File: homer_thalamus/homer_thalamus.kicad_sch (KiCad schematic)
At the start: 20 parts, among them J1 GPIO, J2 MotDrv_Pow_Conn, J3 Right_Motor_Conn, J4 Left_Motor_Conn, J5 Spare_GP_Conn, J6 VBUS_Conn, SW1 SW_PULLDOWN, U1 DRV8874_CARRIER_RIGHT, U2 DRV8874_CARRIER_LEFT, U3 HC-SR04

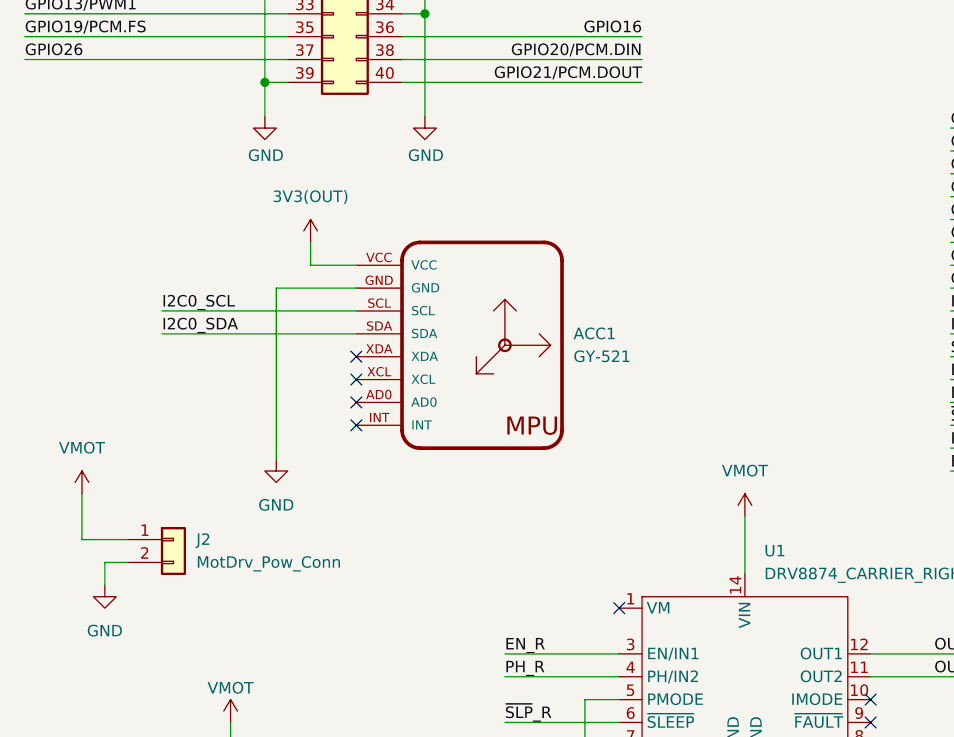
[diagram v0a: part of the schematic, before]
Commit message: update pcb layout
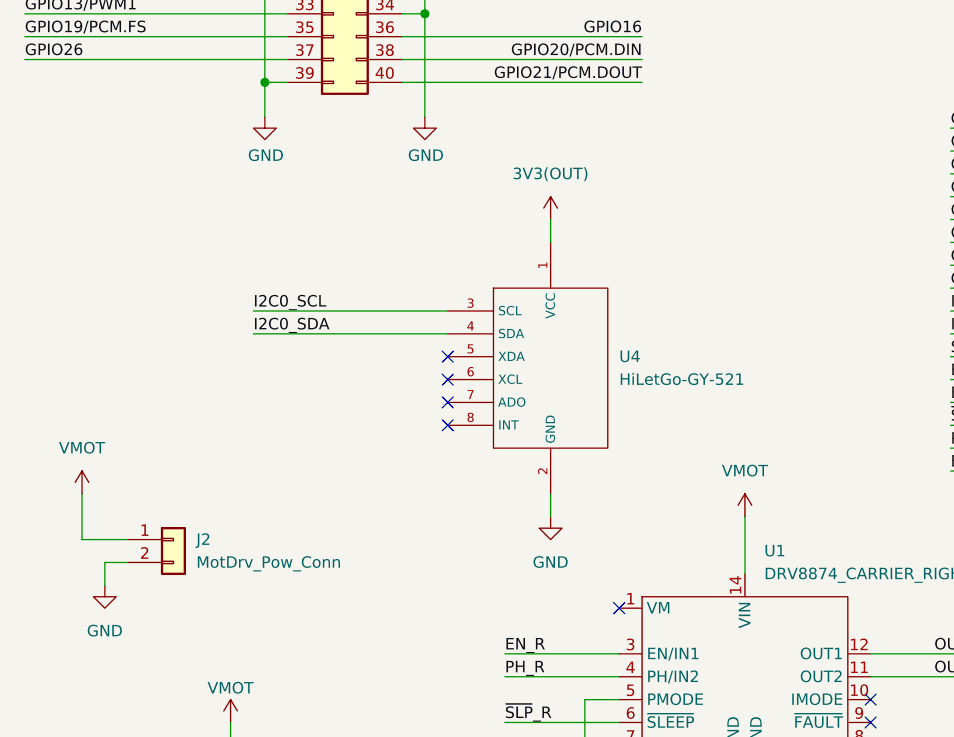
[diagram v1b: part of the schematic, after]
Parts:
- removed ACC1: GY-521, GY-521:GY-521, symbol GY-521:GY-521
- added U4: HiLetGo-GY-521, GY-521:HiLetGo-GY-521, symbol GY-521:HiLetGo-GY-521
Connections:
- net 3V3(OUT): now also U4.1 (VCC)
- net GND: now also U4.2 (GND)
- net I2C0_SCL: now also U4.3 (SCL)
- net I2C0_SDA: now also U4.4 (SDA)
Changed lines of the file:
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@@
 	)
 	(no_connect
-		(at 58.42 111.76)
+		(at 68.58 111.76)
 	)
 	(no_connect
@@
 	)
 	(no_connect
-		(at 58.42 109.22)
+		(at 68.58 109.22)
 	)
 	(no_connect
@@
 	)
 	(no_connect
-		(at 58.42 104.14)
+		(at 68.58 104.14)
 	)
 	(no_connect
@@
 	)
 	(no_connect
-		(at 58.42 106.68)
+		(at 68.58 106.68)
 	)
 	(no_connect
@@
 	(wire
 		(pts
-			(xy 58.42 96.52) (xy 49.53 96.52)
-		)
-		(stroke
-			(width 0)
-			(type default)
-		)
-	)
-	(wire
-		(pts
 			(xy 63.5 53.34) (xy 90.17 53.34)
 		)
@@
 	(wire
 		(pts
-			(xy 49.53 96.52) (xy 49.53 115.57)
-		)
-		(stroke
-			(width 0)
-			(type default)
-		)
-	)
-	(wire
-		(pts
 			(xy 21.59 60.96) (xy 50.8 60.96)
 		)
@@
 	(wire
 		(pts
-			(xy 36.83 99.06) (xy 58.42 99.06)
+			(xy 46.99 99.06) (xy 68.58 99.06)
 		)
 		(stroke
@@
 	(wire
 		(pts
+			(xy 80.01 119.38) (xy 80.01 121.92)
+		)
+		(stroke
+			(width 0)
+			(type default)
+		)
+	)
+	(wire
+		(pts
 			(xy 45.72 21.59) (xy 45.72 25.4)
 		)
@@
 	(wire
 		(pts
-			(xy 36.83 101.6) (xy 58.42 101.6)
+			(xy 46.99 101.6) (xy 68.58 101.6)
 		)
 		(stroke
@@
 	(wire
 		(pts
+			(xy 80.01 88.9) (xy 80.01 91.44)
+		)
+		(stroke
+			(width 0)
+			(type default)
+		)
+	)
+	(wire
+		(pts
 			(xy 43.18 172.72) (xy 43.18 175.26)
 		)
@@
 	(wire
 		(pts
-			(xy 53.34 93.98) (xy 58.42 93.98)
-		)
-		(stroke
-			(width 0)
-			(type default)
-		)
-	)
-	(wire
-		(pts
 			(xy 21.59 68.58) (xy 50.8 68.58)
 		)
@@
 	(wire
 		(pts
-			(xy 53.34 91.44) (xy 53.34 93.98)
-		)
-		(stroke
-			(width 0)
-			(type default)
-		)
-	)
-	(wire
-		(pts
 			(xy 83.82 153.67) (xy 100.33 153.67)
 		)
@@
 	)
 	(label "I2C0_SDA"
-		(at 36.83 101.6 0)
+		(at 46.99 101.6 0)
 		(effects
 			(font
@@
 	)
 	(label "I2C0_SCL"
-		(at 36.83 99.06 0)
+		(at 46.99 99.06 0)
 		(effects
 			(font
@@
 		(lib_name "GND_1")
 		(lib_id "power:GND")
-		(at 49.53 115.57 0)
+		(at 80.01 121.92 0)
 		(unit 1)
 		(exclude_from_sim no)
@@
 		(fields_autoplaced yes)
 		(property "Reference" "#PWR025"
-			(at 49.53 121.92 0)
+			(at 80.01 128.27 0)
 			(effects
 				(font
@@
 		)
 		(property "Value" "GND"
-			(at 49.53 120.65 0)
+			(at 80.01 127 0)
 			(effects
 				(font
@@
 		)
 		(property "Footprint" ""
-			(at 49.53 115.57 0)
+			(at 80.01 121.92 0)
 			(effects
 				(font
@@
 		)
 		(property "Datasheet" ""
-			(at 49.53 115.57 0)
+			(at 80.01 121.92 0)
 			(effects
 				(font
@@
 		)
 		(property "Description" "Power symbol creates a global label with name \"GND\" , ground"
-			(at 49.53 115.57 0)
+			(at 80.01 121.92 0)
 			(effects
 				(font
@@
 	)
 	(symbol
+		(lib_id "GY-521:HiLetGo-GY-521")
+		(at 80.01 105.41 0)
+		(unit 1)
+		(exclude_from_sim no)
+		(in_bom yes)
+		(on_board yes)
+		(dnp no)
+		(fields_autoplaced yes)
+		(property "Reference" "U4"
+			(at 87.63 104.1399 0)
+			(effects
+				(font
+					(size 1.27 1.27)
+				)
+				(justify left)
+			)
+		)
+		(property "Value" "HiLetGo-GY-521"
+			(at 87.63 106.6799 0)
+			(effects
+				(font
+					(size 1.27 1.27)
+				)
+				(justify left)
+			)
+		)
+		(property "Footprint" "GY-521:HiLetGo-GY-521"
+			(at 81.28 105.41 0)
+			(effects
+				(font
+					(size 1.27 1.27)
+				)
+				(hide yes)
+			)
+		)
+		(property "Datasheet" ""
+			(at 81.28 105.41 0)
+			(effects
+				(font
+					(size 1.27 1.27)
+				)
+				(hide yes)
+			)
+		)
+		(property "Description" ""
+			(at 81.28 105.41 0)
+			(effects
+				(font
+					(size 1.27 1.27)
+				)
+				(hide yes)
+			)
+		)
+		(pin "2"
+		)
+		(pin "8"
+		)
+		(pin "1"
+		)
+		(pin "6"
+		)
+		(pin "4"
+		)
+		(pin "3"
+		)
+		(pin "5"
+		)
+		(pin "7"
+		)
+		(instances
+			(project ""
+				(path "/e63e39d7-6ac0-4ffd-8aa3-1841a4541b55"
+					(reference "U4")
+					(unit 1)
+				)
+			)
+		)
+	)
+	(symbol
 		(lib_name "GND_1")
 		(lib_id "power:GND")
@@
 	(symbol
 		(lib_id "power:+3V3")
-		(at 53.34 91.44 0)
+		(at 80.01 88.9 0)
 		(unit 1)
 		(exclude_from_sim no)
@@
 		(fields_autoplaced yes)
 		(property "Reference" "#PWR024"
-			(at 53.34 95.25 0)
+			(at 80.01 92.71 0)
 			(effects
 				(font
@@
 		)
 		(property "Value" "3V3(OUT)"
-			(at 53.34 86.36 0)
+			(at 80.01 83.82 0)
 			(effects
 				(font
@@
 		)
 		(property "Footprint" ""
-			(at 53.34 91.44 0)
+			(at 80.01 88.9 0)
 			(effects
 				(font
@@
 		)
 		(property "Datasheet" ""
-			(at 53.34 91.44 0)
+			(at 80.01 88.9 0)
 			(effects
 				(font
@@
 		)
 		(property "Description" "Power symbol creates a global label with name \"+3V3\""
-			(at 53.34 91.44 0)
+			(at 80.01 88.9 0)
 			(effects
 				(font
@@
 					(unit 1)
 				)
-			)
-		)
-	)
-	(symbol
-		(lib_id "GY-521:GY-521")
-		(at 74.93 102.87 0)
-		(unit 1)
-		(exclude_from_sim no)
-		(in_bom yes)
-		(on_board yes)
-		(dnp no)
-		(fields_autoplaced yes)
-		(property "Reference" "ACC1"
-			(at 82.55 101.5999 0)
-			(effects
-				(font
-					(size 1.27 1.27)
-				)
-				(justify left)
-			)
-		)
-		(property "Value" "GY-521"
-			(at 82.55 104.1399 0)
-			(effects
-				(font
-					(size 1.27 1.27)
-				)
-				(justify left)
-			)
-		)
-		(property "Footprint" "GY-521:GY-521"
-			(at 74.93 102.87 0)
-			(effects
-				(font
-					(size 1.27 1.27)
-				)
-				(hide yes)
-			)
-		)
-		(property "Datasheet" ""
-			(at 74.93 102.87 0)
-			(effects
-				(font
-					(size 1.27 1.27)
-				)
-				(hide yes)
-			)
-		)
-		(property "Description" ""
-			(at 74.93 102.87 0)
-			(effects
-				(font
-					(size 1.27 1.27)
-				)
-				(hide yes)
-			)
-		)
-		(property "MF" "GODREAM FORDREAM CO., LIMITED"
-			(at 74.93 102.87 0)
-			(effects
-				(font
-					(size 1.27 1.27)
-				)
-				(justify bottom)
-				(hide yes)
-			)
-		)
-		(property "Description_1" "Triple Axis Accelerometer Gyro Breakout"
-			(at 74.93 102.87 0)
-			(effects
-				(font
-					(size 1.27 1.27)
-				)
-				(justify bottom)
-				(hide yes)
-			)
-		)
-		(property "Package" "Package"
-			(at 74.93 102.87 0)
-			(effects
-				(font
-					(size 1.27 1.27)
-				)
-				(justify bottom)
-				(hide yes)
-			)
-		)
-		(property "Price" "None"
-			(at 74.93 102.87 0)
-			(effects
-				(font
-					(size 1.27 1.27)
-				)
-				(justify bottom)
-				(hide yes)
-			)
-		)
-		(property "SnapEDA_Link" "https://www.snapeda.com/parts/GY-521/GODREAM+FORDREAM+CO.%252C+LIMITED/view-part/?ref=snap"
-			(at 74.93 102.87 0)
-			(effects
-				(font
-					(size 1.27 1.27)
-				)
-				(justify bottom)
-				(hide yes)
-			)
-		)
-		(property "MP" "GY-521"
-			(at 74.93 102.87 0)
-			(effects
-				(font
-					(size 1.27 1.27)
-				)
-				(justify bottom)
-				(hide yes)
-			)
-		)
-		(property "Availability" "Not in stock"
-			(at 74.93 102.87 0)
-			(effects
-				(font
-					(size 1.27 1.27)
-				)
-				(justify bottom)
-				(hide yes)
-			)
-		)
-		(property "Check_prices" "https://www.snapeda.com/parts/GY-521/GODREAM+FORDREAM+CO.%252C+LIMITED/view-part/?ref=eda"
-			(at 74.93 102.87 0)
-			(effects
-				(font
-					(size 1.27 1.27)
-				)
-				(justify bottom)
-				(hide yes)
-			)
-		)
-		(pin "XCL"
-		)
-		(pin "XDA"
-		)
-		(pin "INT"
-		)
-		(pin "SDA"
-		)
-		(pin "AD0"
-		)
-		(pin "SCL"
-		)
-		(pin "GND"
-		)
-		(pin "VCC"
-		)
-		(instances
-			(project ""
-				(path "/e63e39d7-6ac0-4ffd-8aa3-1841a4541b55"
-					(reference "ACC1")
-					(unit 1)
-				)
